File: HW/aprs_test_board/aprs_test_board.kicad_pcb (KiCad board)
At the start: 2 copper layers, 48.4 x 25.5 mm, 23 parts, among them J1 Conn_Coaxial, J2 Conn_01x06, J3 Conn_01x06, U1 Si4461, Y1 30M

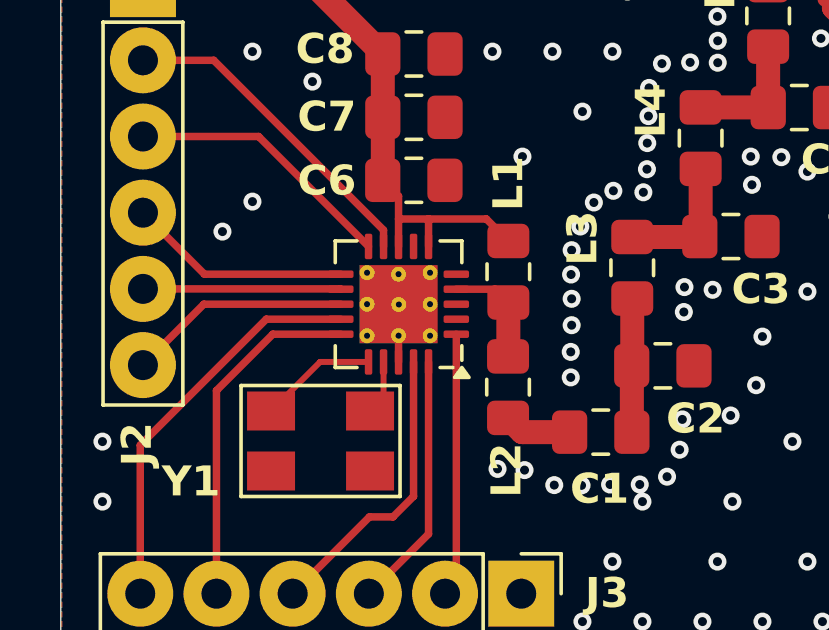
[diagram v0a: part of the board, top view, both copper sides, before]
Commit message: little fix
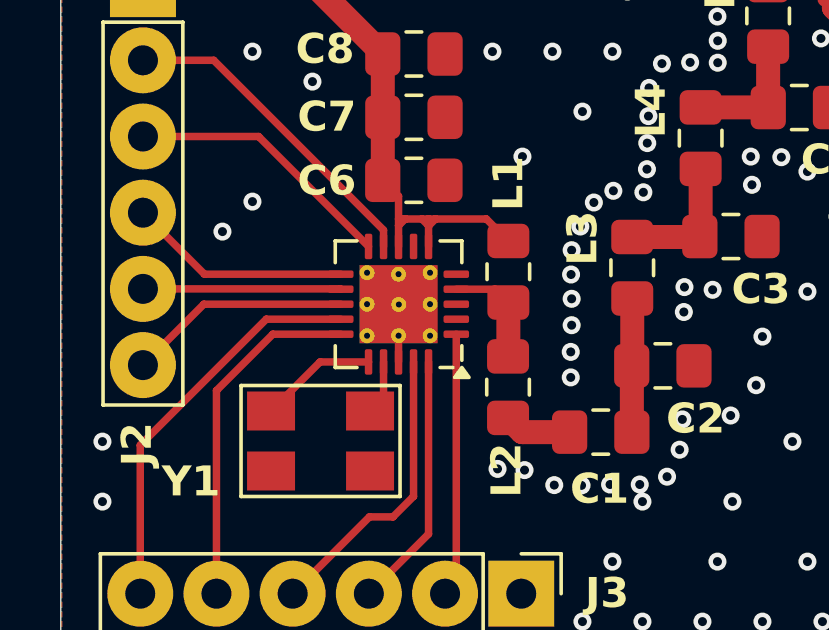
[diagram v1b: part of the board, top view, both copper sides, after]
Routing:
- net +3.3V: track 20.6 -> 21.5 mm
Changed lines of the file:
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@@
 	)
 	(segment
-		(start 101.87 100.58)
-		(end 103.7975 100.58)
-		(width 0.25)
-		(layer "F.Cu")
-		(net 7)
-	)
-	(segment
-		(start 101.87 100.58)
-		(end 100.87 100.58)
+		(start 101.87 100.8)
+		(end 101.87 100.58)
 		(width 0.25)
 		(layer "F.Cu")
@@
 	)
 	(segment
+		(start 102.1 100.58)
+		(end 103.7975 100.58)
+		(width 0.25)
+		(layer "F.Cu")
+		(net 7)
+	)
+	(segment
 		(start 100.345 99.2875)
 		(end 100.3425 99.29)
@@
 	)
 	(segment
+		(start 101.87 100.8)
+		(end 101.88 100.8)
+		(width 0.25)
+		(layer "F.Cu")
+		(net 7)
+	)
+	(segment
 		(start 97.775 92.51)
 		(end 100.345 95.08)
@@
 	)
 	(segment
+		(start 101.1 100.58)
+		(end 100.87 100.58)
+		(width 0.25)
+		(layer "F.Cu")
+		(net 7)
+	)
+	(segment
 		(start 100.345 95.08)
 		(end 100.345 97.19)
@@
 	)
 	(segment
+		(start 101.88 100.8)
+		(end 102.1 100.58)
+		(width 0.25)
+		(layer "F.Cu")
+		(net 7)
+	)
+	(segment
+		(start 101.65 100.58)
+		(end 101.1 100.58)
+		(width 0.25)
+		(layer "F.Cu")
+		(net 7)
+	)
+	(segment
+		(start 101.87 100.58)
+		(end 102.1 100.58)
+		(width 0.25)
+		(layer "F.Cu")
+		(net 7)
+	)
+	(segment
 		(start 92.35 92.51)
 		(end 97.775 92.51)
@@
 	)
 	(segment
+		(start 101.09 100.58)
+		(end 100.87 100.8)
+		(width 0.25)
+		(layer "F.Cu")
+		(net 7)
+	)
+	(segment
+		(start 101.1 100.58)
+		(end 101.09 100.58)
+		(width 0.25)
+		(layer "F.Cu")
+		(net 7)
+	)
+	(segment
 		(start 101.87 101.495)
-		(end 101.87 100.58)
+		(end 101.87 100.8)
+		(width 0.25)
+		(layer "F.Cu")
+		(net 7)
+	)
+	(segment
+		(start 101.87 100.58)
+		(end 101.65 100.58)
 		(width 0.25)
 		(layer "F.Cu")
@@
 	)
 	(segment
+		(start 100.87 100.8)
+		(end 100.87 100.58)
+		(width 0.25)
+		(layer "F.Cu")
+		(net 7)
+	)
+	(segment
+		(start 101.87 100.8)
+		(end 101.65 100.58)
+		(width 0.25)
+		(layer "F.Cu")
+		(net 7)
+	)
+	(segment
 		(start 100.87 101.495)
-		(end 100.87 100.58)
+		(end 100.87 100.8)
 		(width 0.25)
 		(layer "F.Cu")
@@
 		(start 100.37 105.345)
 		(end 100.37 106.53)
-		(width 0.2)
+		(width 0.25)
 		(layer "F.Cu")
 		(net 17)
@@
 		(start 99.87 105.345)
 		(end 98.255 105.345)
-		(width 0.2)
+		(width 0.25)
 		(layer "F.Cu")
 		(net 18)
@@
 		(start 98.255 105.345)
 		(end 96.62 106.98)
-		(width 0.2)
+		(width 0.25)
 		(layer "F.Cu")
 		(net 18)
